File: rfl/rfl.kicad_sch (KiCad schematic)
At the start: 37 parts, among them J1 636101111001, J2 Conn_01x09, J801 629722000214, J802 swd, U1 SX1281, U2 STM32G0B1KETxN, U3 TPS7A19, U801 USBLC6-2SC6, Y1 52MHz

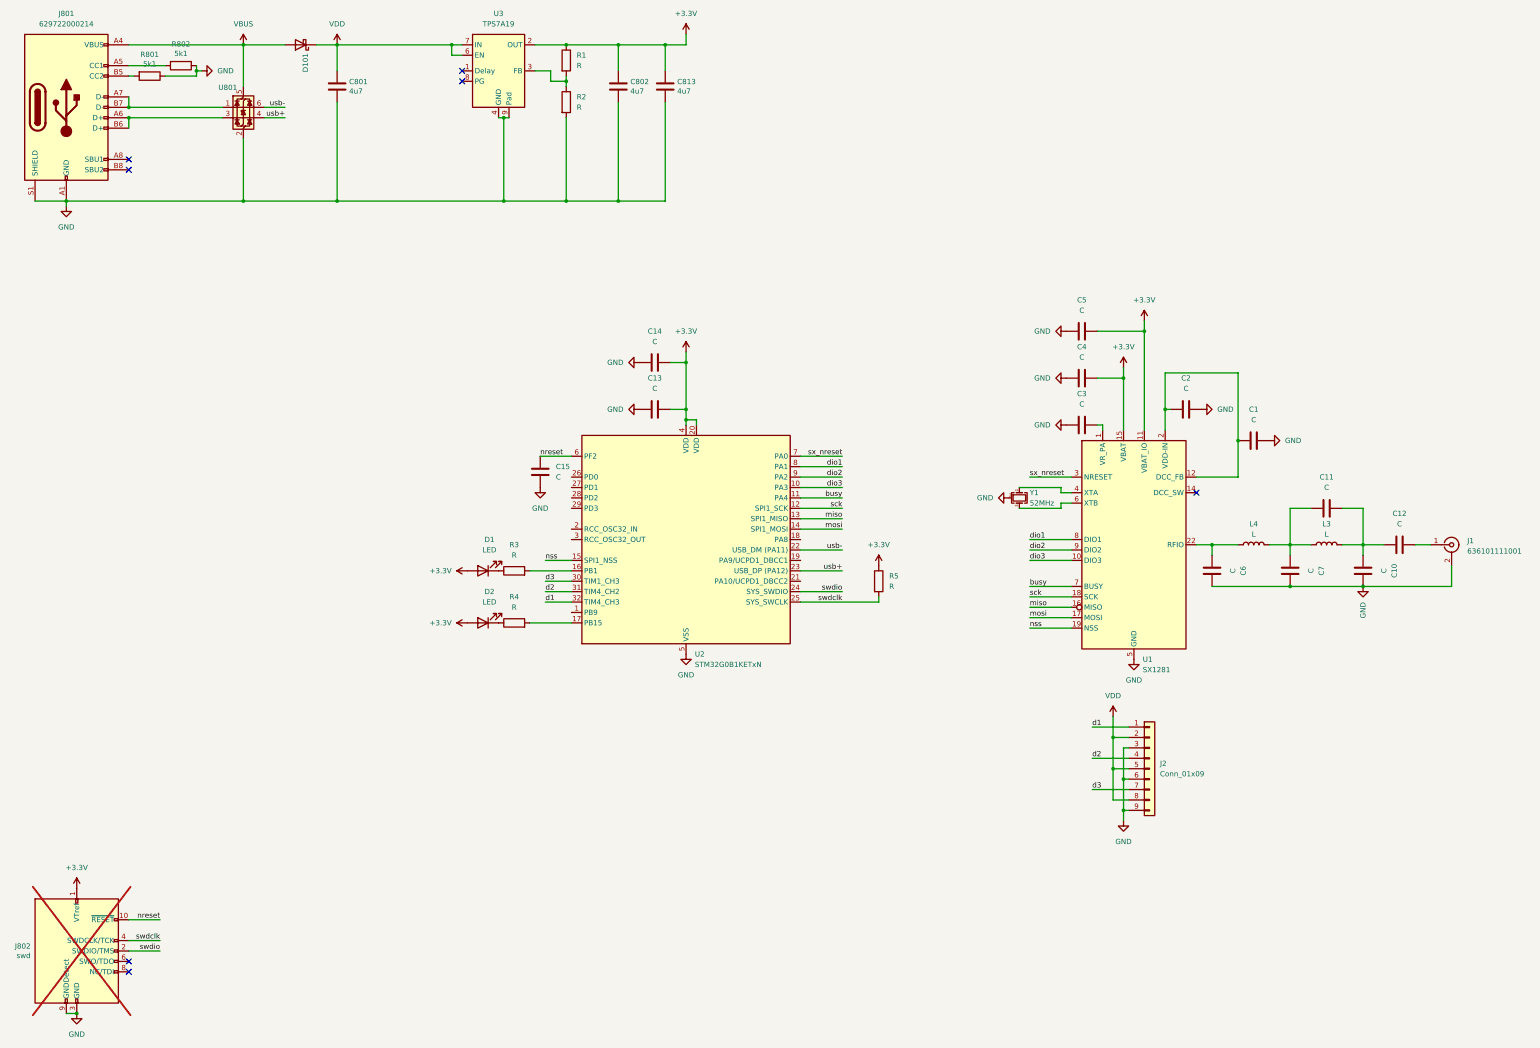
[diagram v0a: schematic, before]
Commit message: v2 with rf switch wip
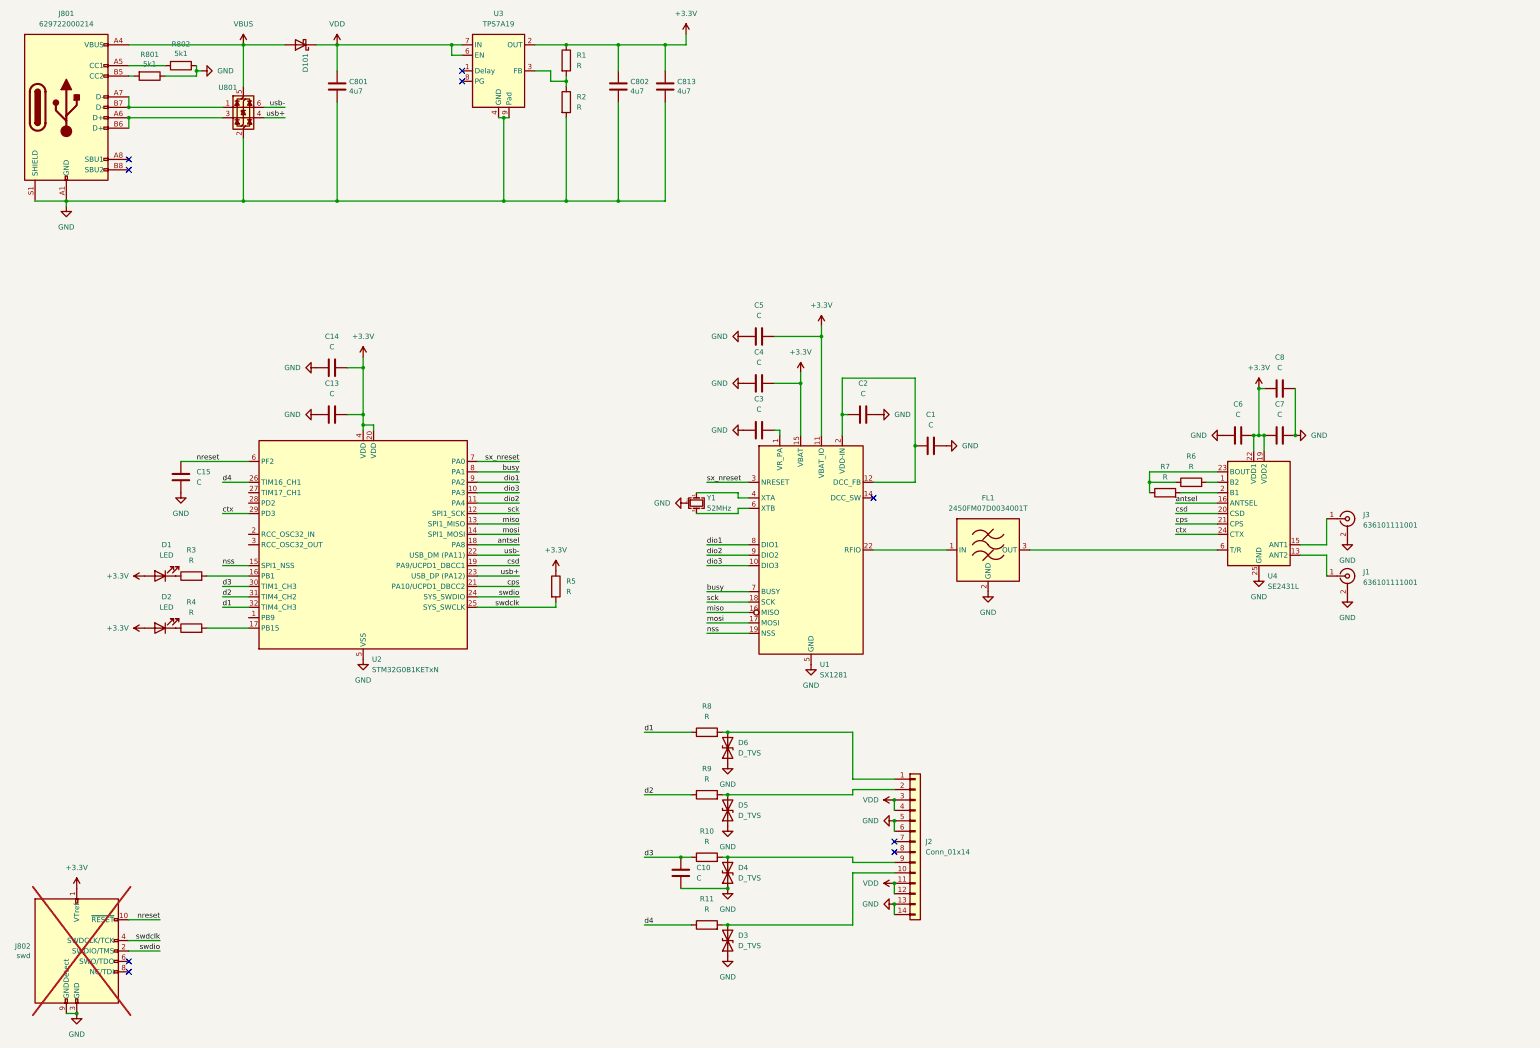
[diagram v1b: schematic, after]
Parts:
- removed C11, C12: C, Capacitor_SMD:C_0402_1005Metric, symbol Device:C
- removed J2: Conn_01x09, Connector_PinHeader_2.54mm:PinHeader_1x09_P2.54mm_Horizontal, symbol Connector_Generic:Conn_01x09
- removed L3, L4: L, Inductor_SMD:L_0402_1005Metric, symbol Device:L
- added C8: C, Capacitor_SMD:C_0603_1608Metric, symbol Device:C
- added D3, D4, D5, D6: D_TVS, Diode_SMD:D_0402_1005Metric, symbol Device:D_TVS
- added FL1: 2450FM07D0034001T, rfl-lib-fp:2450FM07D0034001T, symbol RF_Filter:BFCN-2450
- added J2: Conn_01x14, rfl-lib-fp:PinHeader_2x07_P2.54mm_Edge, symbol Connector_Generic:Conn_01x14
- added J3: 636101111001, Connector_Coaxial:U.FL_Hirose_U.FL-R-SMT-1_Vertical, symbol Connector:Conn_Coaxial
- added R10, R11, R6, R7, R8, R9: R, Resistor_SMD:R_0402_1005Metric, symbol Device:R
- added U4: SE2431L, Package_DFN_QFN:QFN-24-1EP_3x4mm_P0.4mm_EP1.65x2.65mm, symbol rfl_lib:SE2431L
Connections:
- net +3.3V: now also C6.2, C7.1, C8.1, U4.19 (VDD2), U4.22 (VDD1)
- net GND: now also C10.1, C6.1, C8.2, D3.1 (A1), D4.1 (A1), D5.1 (A1), D6.1 (A1), FL1.2 (GND), FL1.4 (GND), J2.13 (Pin_13), J2.14 (Pin_14), J2.5 (Pin_5), J2.6 (Pin_6), J3.2 (Ext), U4.10 (GND), U4.11 (GND), U4.12 (GND), U4.14 (GND), U4.18 (GND), U4.25 (GND), U4.9 (GND); no longer C10.2, C6.2
- net VDD: now also J2.11 (Pin_11), J2.12 (Pin_12), J2.3 (Pin_3), J2.4 (Pin_4)
- net busy: now also U2.8 (PA1); no longer U2.11 (PA4)
- net d1: now also R8.1
- net d2: now also R9.1
- net d3: now also C10.2, R10.1
- net dio1: now also U2.9 (PA2); no longer U2.8 (PA1)
- net dio2: now also U2.11 (PA4); no longer U2.9 (PA2)
- net at U1.22 (RFIO): now also FL1.1 (IN); no longer C6.1
- net at J1.1 (In): now also U4.13 (ANT2)
- net antsel: now reaches U2.18 (PA8)
- net antsel: now also U4.16 (ANTSEL)
- net csd: now reaches U2.19 (PA9/UCPD1_DBCC1)
- net csd: now also U4.20 (CSD)
- net cps: now reaches U2.21 (PA10/UCPD1_DBCC2)
- net cps: now also U4.21 (CPS)
- net d4: now reaches U2.26 (PD0)
- net d4: now also R11.1
- net ctx: now reaches U2.29 (PD3)
- net ctx: now also U4.24 (CTX)
- new net: R6.2, U4.1 (B2)
- new net: J3.1 (In), U4.15 (ANT1)
- new net: R7.2, U4.2 (B1)
- new net: R6.1, R7.1, U4.23 (BOUT)
- new net: FL1.3 (OUT), U4.6 (T/R)
- new net: D6.2 (A2), J2.1 (Pin_1), R8.2
- new net: D4.2 (A2), J2.9 (Pin_9), R10.2
- new net: D3.2 (A2), J2.10 (Pin_10), R11.2
- new net: D5.2 (A2), J2.2 (Pin_2), R9.2
- no-connect marks 7 -> 9
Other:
- moved on the sheet: C1, C13, C14, C15, C2, C3, C4, C5, D1, D2, J1, R3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

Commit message: fixed edge cleareance
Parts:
- J801: footprint et-misc:USB_C_Receptacle_GCT_USB4105-xx-A_16P_TopMnt_Horizontal -> rfl-lib-fp:USB_C_Receptacle_GCT_USB4105-xx-A_16P_TopMnt_Horizontal
- J802: footprint et-misc:PinHeader_2x05_P1.27mm_Vertical_SMD -> Connector_PinHeader_1.27mm:PinHeader_2x05_P1.27mm_Vertical_SMD
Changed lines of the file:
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@@
 			)
 		)
-		(property "Footprint" "et-misc:USB_C_Receptacle_GCT_USB4105-xx-A_16P_TopMnt_Horizontal"
+		(property "Footprint" "rfl-lib-fp:USB_C_Receptacle_GCT_USB4105-xx-A_16P_TopMnt_Horizontal"
 			(at 43.18 48.26 0)
 			(hide yes)
@@
 			)
 		)
-		(property "Footprint" "et-misc:PinHeader_2x05_P1.27mm_Vertical_SMD"
+		(property "Footprint" "Connector_PinHeader_1.27mm:PinHeader_2x05_P1.27mm_Vertical_SMD"
 			(at 41.91 254 0)
 			(hide yes)
